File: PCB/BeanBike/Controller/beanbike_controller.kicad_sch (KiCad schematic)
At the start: 16 parts, among them SW1 SW_Push, U4 STM32G473RETx, X1 X49SM8MSD2SC

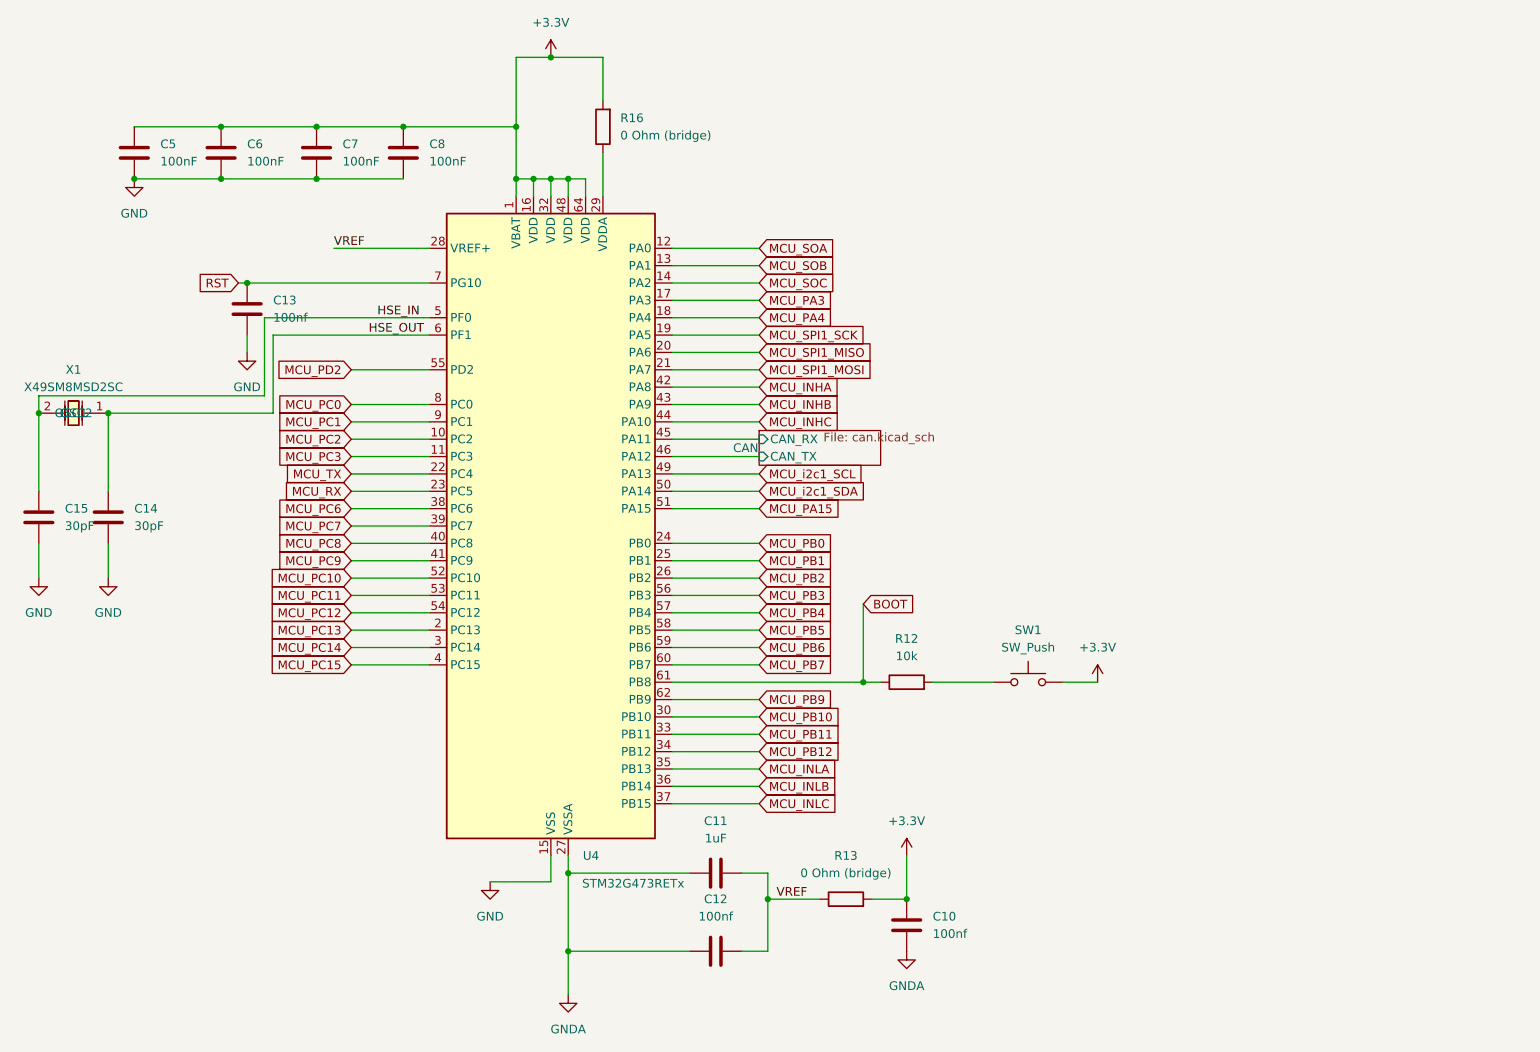
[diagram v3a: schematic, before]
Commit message: PCB v3
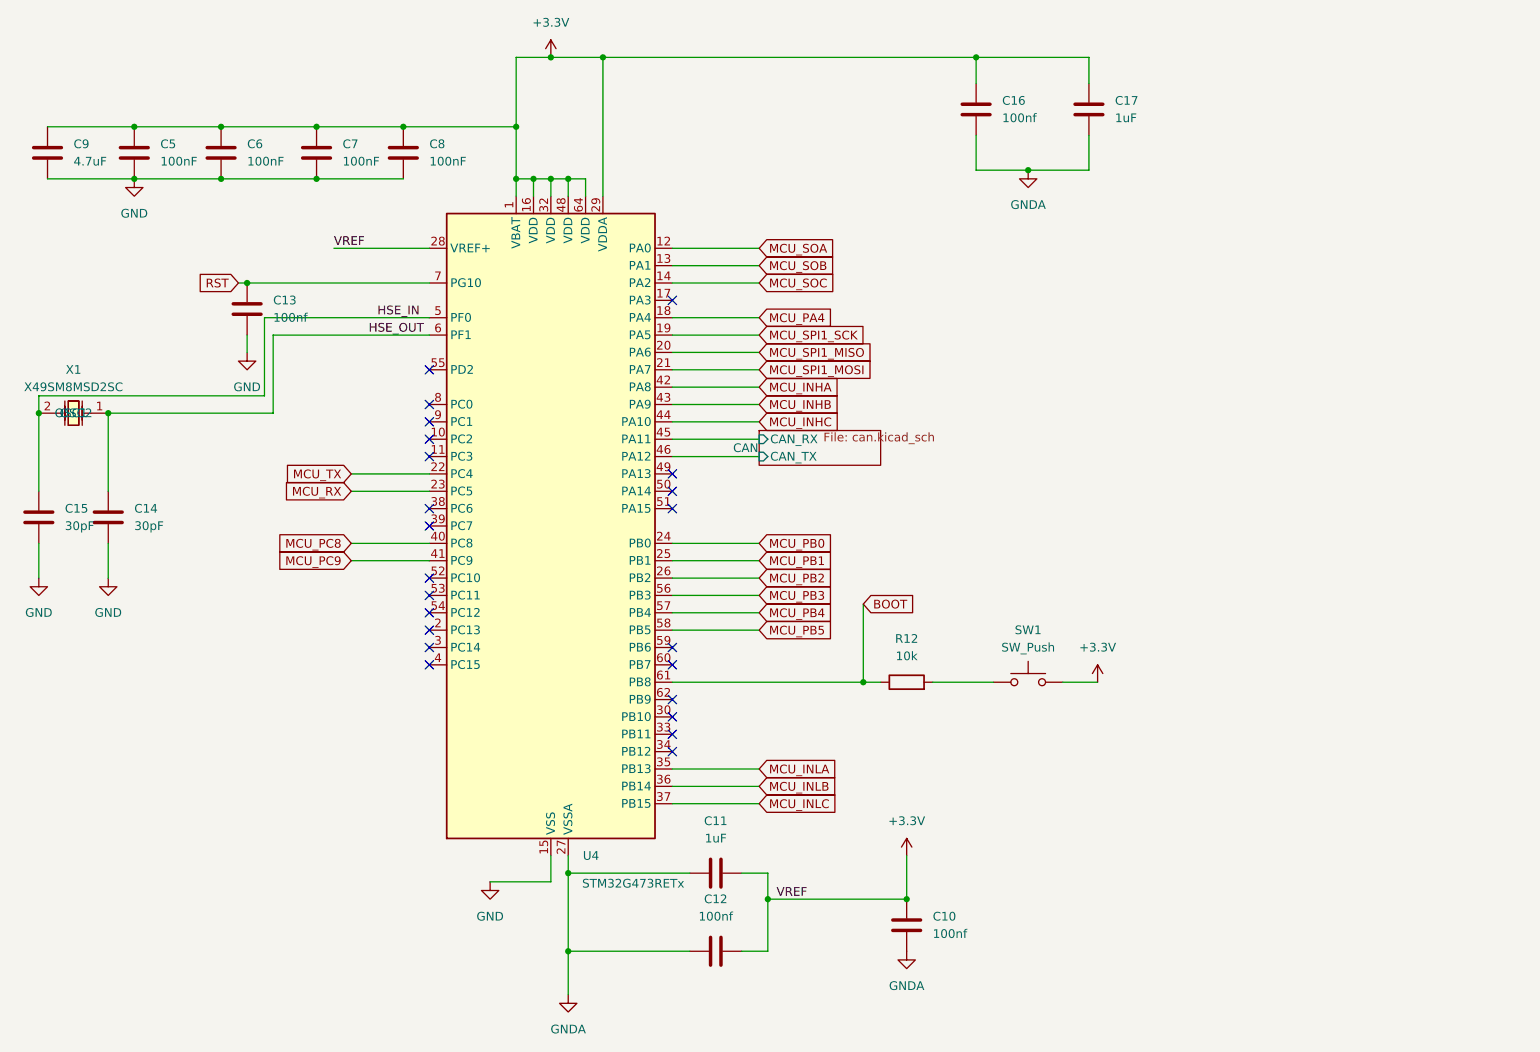
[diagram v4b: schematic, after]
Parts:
- removed R13, R16: 0 Ohm (bridge), Resistor_SMD:R_0805_2012Metric, symbol Device:R
- added C16: 100nf, Capacitor_SMD:C_0402_1005Metric, symbol Device:C
- added C17: 1uF, Capacitor_SMD:C_0402_1005Metric, symbol Device:C
- added C9: 4.7uF, Capacitor_SMD:C_0402_1005Metric, symbol Device:C
- U4: LCSC (none) -> C730120
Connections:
- net VREF is gone; now on net +3.3V: C11.2, C12.2, U4.28 (VREF+)
- net +3.3V: now also U4.29 (VDDA), C16.1, C17.1, C9.1
- net GND: now also C9.2
- net GNDA: now also C16.2, C17.2
- net MCU_PA15: no longer names the net of U4.51 (PA15)
- net MCU_PA3: no longer names the net of U4.17 (PA3)
- net MCU_PB10: no longer names the net of U4.30 (PB10)
- net MCU_PB11: no longer names the net of U4.33 (PB11)
- net MCU_PB12: no longer names the net of U4.34 (PB12)
- net MCU_PB6: no longer names the net of U4.59 (PB6)
- net MCU_PB7: no longer names the net of U4.60 (PB7)
- net MCU_PB9: no longer names the net of U4.62 (PB9)
- net MCU_PC0: no longer names the net of U4.8 (PC0)
- net MCU_PC1: no longer names the net of U4.9 (PC1)
- net MCU_PC10: no longer names the net of U4.52 (PC10)
- net MCU_PC11: no longer names the net of U4.53 (PC11)
- net MCU_PC12: no longer names the net of U4.54 (PC12)
- net MCU_PC13: no longer names the net of U4.2 (PC13)
- net MCU_PC14: no longer names the net of U4.3 (PC14)
- net MCU_PC15: no longer names the net of U4.4 (PC15)
- net MCU_PC2: no longer names the net of U4.10 (PC2)
- net MCU_PC3: no longer names the net of U4.11 (PC3)
- net MCU_PC6: no longer names the net of U4.38 (PC6)
- net MCU_PC7: no longer names the net of U4.39 (PC7)
- net MCU_PD2: no longer names the net of U4.55 (PD2)
- net MCU_i2c1_SCL: no longer names the net of U4.49 (PA13)
- net MCU_i2c1_SDA: no longer names the net of U4.50 (PA14)
- no-connect marks 0 -> 23

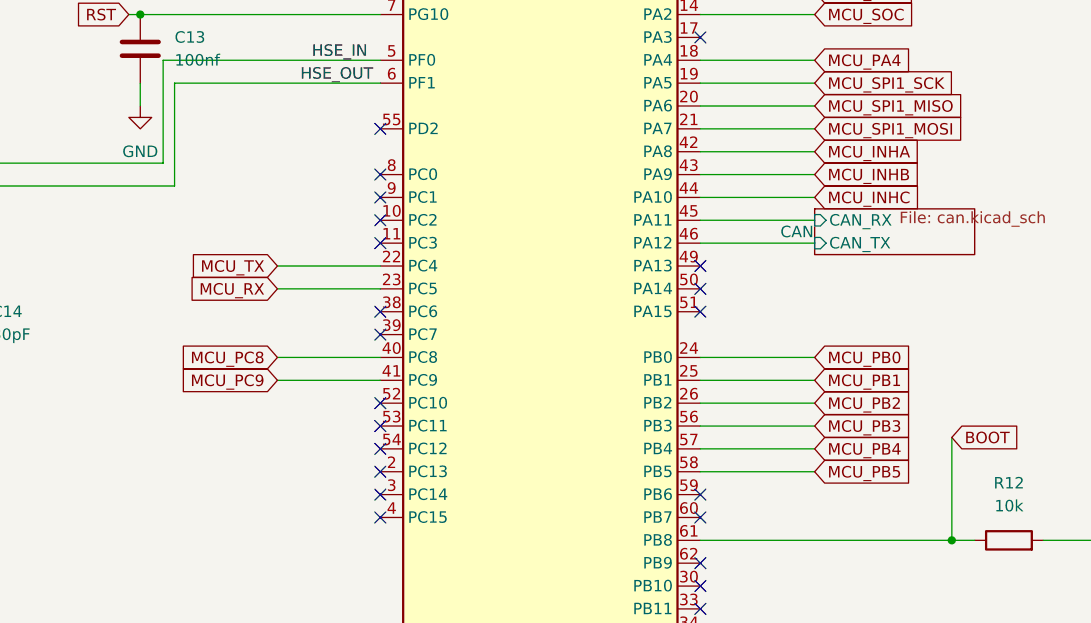
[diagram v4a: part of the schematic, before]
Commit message: PCB v3
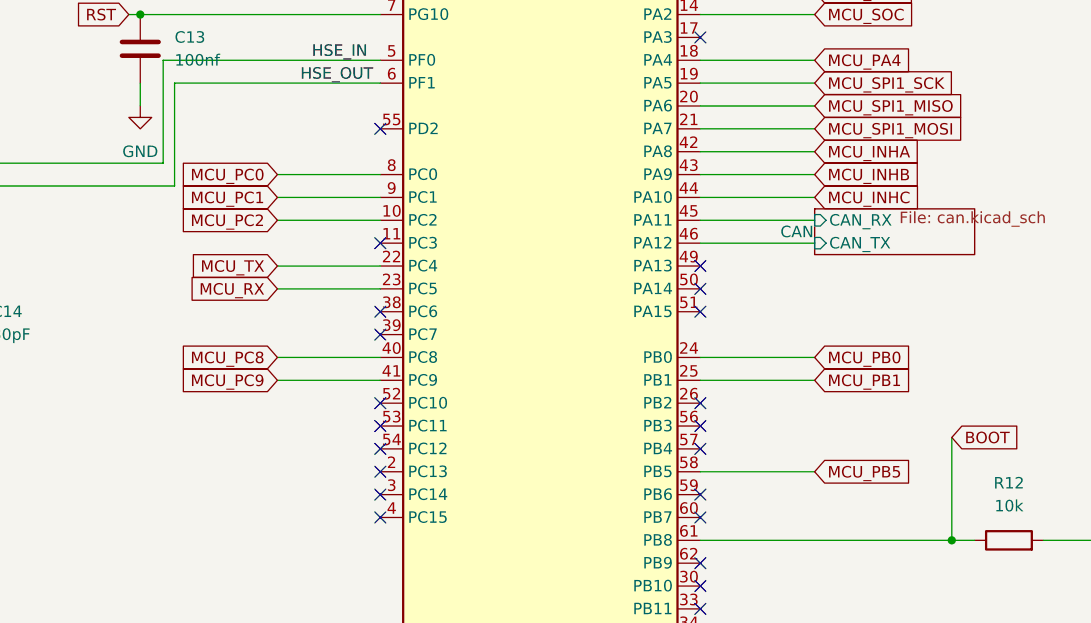
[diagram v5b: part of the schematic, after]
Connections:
- net MCU_PC2: now reaches U4.10 (PC2)
- net MCU_PC0: now reaches U4.8 (PC0)
- net MCU_PC1: now reaches U4.9 (PC1)
- net MCU_PB2: no longer names the net of U4.26 (PB2)
- net MCU_PB3: no longer names the net of U4.56 (PB3)
- net MCU_PB4: no longer names the net of U4.57 (PB4)
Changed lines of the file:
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@@
 	)
 	(no_connect
-		(at 119.38 82.55)
+		(at 154.94 107.95)
+	)
+	(no_connect
+		(at 154.94 110.49)
 	)
 	(no_connect
@@
 	)
 	(no_connect
-		(at 119.38 87.63)
-	)
-	(no_connect
 		(at 154.94 130.81)
 	)
@@
 	)
 	(no_connect
-		(at 119.38 85.09)
+		(at 154.94 113.03)
 	)
 	(no_connect
@@
 	(wire
 		(pts
+			(xy 107.95 82.55) (xy 119.38 82.55)
+		)
+		(stroke
+			(width 0)
+			(type default)
+		)
+	)
+	(wire
+		(pts
 			(xy 168.91 162.56) (xy 168.91 154.94)
 		)
@@
 	(wire
 		(pts
-			(xy 154.94 110.49) (xy 167.64 110.49)
-		)
-		(stroke
-			(width 0)
-			(type default)
-		)
-	)
-	(wire
-		(pts
 			(xy 154.94 140.97) (xy 167.64 140.97)
 		)
@@
 	(wire
 		(pts
+			(xy 107.95 85.09) (xy 119.38 85.09)
+		)
+		(stroke
+			(width 0)
+			(type default)
+		)
+	)
+	(wire
+		(pts
 			(xy 139.7 151.13) (xy 157.48 151.13)
 		)
@@
 	(wire
 		(pts
+			(xy 107.95 87.63) (xy 119.38 87.63)
+		)
+		(stroke
+			(width 0)
+			(type default)
+		)
+	)
+	(wire
+		(pts
 			(xy 134.62 49.53) (xy 132.08 49.53)
 		)
@@
 	(wire
 		(pts
-			(xy 154.94 107.95) (xy 167.64 107.95)
-		)
-		(stroke
-			(width 0)
-			(type default)
-		)
-	)
-	(wire
-		(pts
 			(xy 88.9 49.53) (xy 102.87 49.53)
 		)
@@
 		(pts
 			(xy 132.08 41.91) (xy 132.08 49.53)
-		)
-		(stroke
-			(width 0)
-			(type default)
-		)
-	)
-	(wire
-		(pts
-			(xy 154.94 113.03) (xy 167.64 113.03)
 		)
 		(stroke
@@
 		)
 	)
-	(global_label "MCU_PB3"
-		(shape input)
-		(at 167.64 110.49 0)
-		(fields_autoplaced yes)
-		(effects
-			(font
-				(size 1.27 1.27)
-			)
-			(justify left)
-		)
-		(property "Intersheetrefs" "${INTERSHEET_REFS}"
-			(at 179.3942 110.49 0)
-			(effects
-				(font
-					(size 1.27 1.27)
-				)
-				(justify left)
-				(hide yes)
-			)
-		)
-	)
 	(global_label "MCU_PC8"
 		(shape input)
@@
 		)
 	)
-	(global_label "MCU_PB4"
-		(shape input)
-		(at 167.64 113.03 0)
-		(fields_autoplaced yes)
-		(effects
-			(font
-				(size 1.27 1.27)
-			)
-			(justify left)
-		)
-		(property "Intersheetrefs" "${INTERSHEET_REFS}"
-			(at 179.3942 113.03 0)
-			(effects
-				(font
-					(size 1.27 1.27)
-				)
-				(justify left)
-				(hide yes)
-			)
-		)
-	)
 	(global_label "MCU_INHC"
 		(shape input)
@@
 		)
 	)
+	(global_label "MCU_PC1"
+		(shape input)
+		(at 107.95 85.09 180)
+		(fields_autoplaced yes)
+		(effects
+			(font
+				(size 1.27 1.27)
+			)
+			(justify right)
+		)
+		(property "Intersheetrefs" "${INTERSHEET_REFS}"
+			(at 96.1958 85.09 0)
+			(effects
+				(font
+					(size 1.27 1.27)
+				)
+				(justify right)
+				(hide yes)
+			)
+		)
+	)
 	(global_label "MCU_PC9"
 		(shape input)
@@
 		)
 	)
-	(global_label "MCU_PB2"
-		(shape input)
-		(at 167.64 107.95 0)
-		(fields_autoplaced yes)
-		(effects
-			(font
-				(size 1.27 1.27)
-			)
-			(justify left)
-		)
-		(property "Intersheetrefs" "${INTERSHEET_REFS}"
-			(at 179.3942 107.95 0)
-			(effects
-				(font
-					(size 1.27 1.27)
-				)
-				(justify left)
-				(hide yes)
-			)
-		)
-	)
 	(global_label "MCU_SOB"
 		(shape input)
@@
 		)
 	)
+	(global_label "MCU_PC0"
+		(shape input)
+		(at 107.95 82.55 180)
+		(fields_autoplaced yes)
+		(effects
+			(font
+				(size 1.27 1.27)
+			)
+			(justify right)
+		)
+		(property "Intersheetrefs" "${INTERSHEET_REFS}"
+			(at 96.1958 82.55 0)
+			(effects
+				(font
+					(size 1.27 1.27)
+				)
+				(justify right)
+				(hide yes)
+			)
+		)
+	)
 	(global_label "MCU_RX"
 		(shape input)
@@
 				(hide yes)
 			)
+		)
+	)
+	(global_label "MCU_PC2"
+		(shape input)
+		(at 107.95 87.63 180)
+		(fields_autoplaced yes)
+		(effects
+			(font
+				(size 1.27 1.27)
+			)
+			(justify right)
+		)
+		(property "Intersheetrefs" "${INTERSHEET_REFS}"
+			(at 96.1958 87.63 0)
+			(effects
+				(font
+					(size 1.27 1.27)
+				)
+				(justify right)
+				(hide yes)
+			)

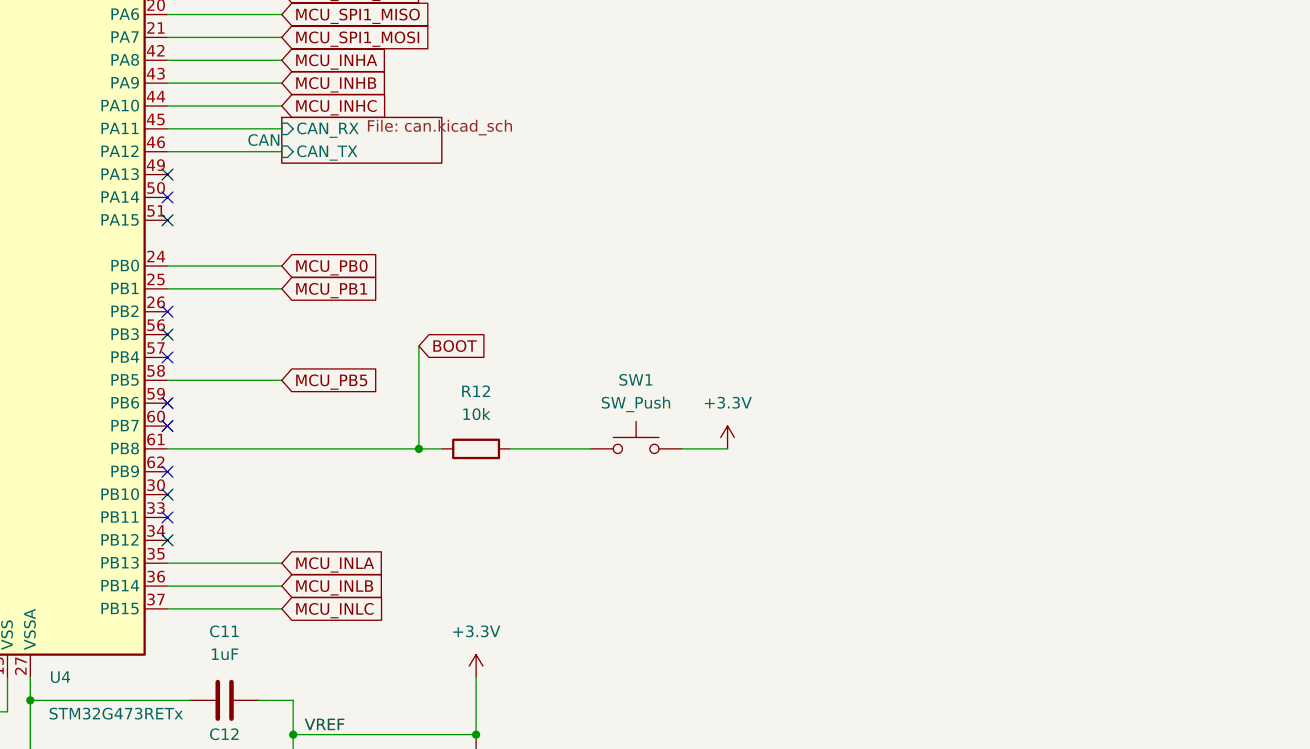
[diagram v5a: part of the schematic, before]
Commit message: big ol update
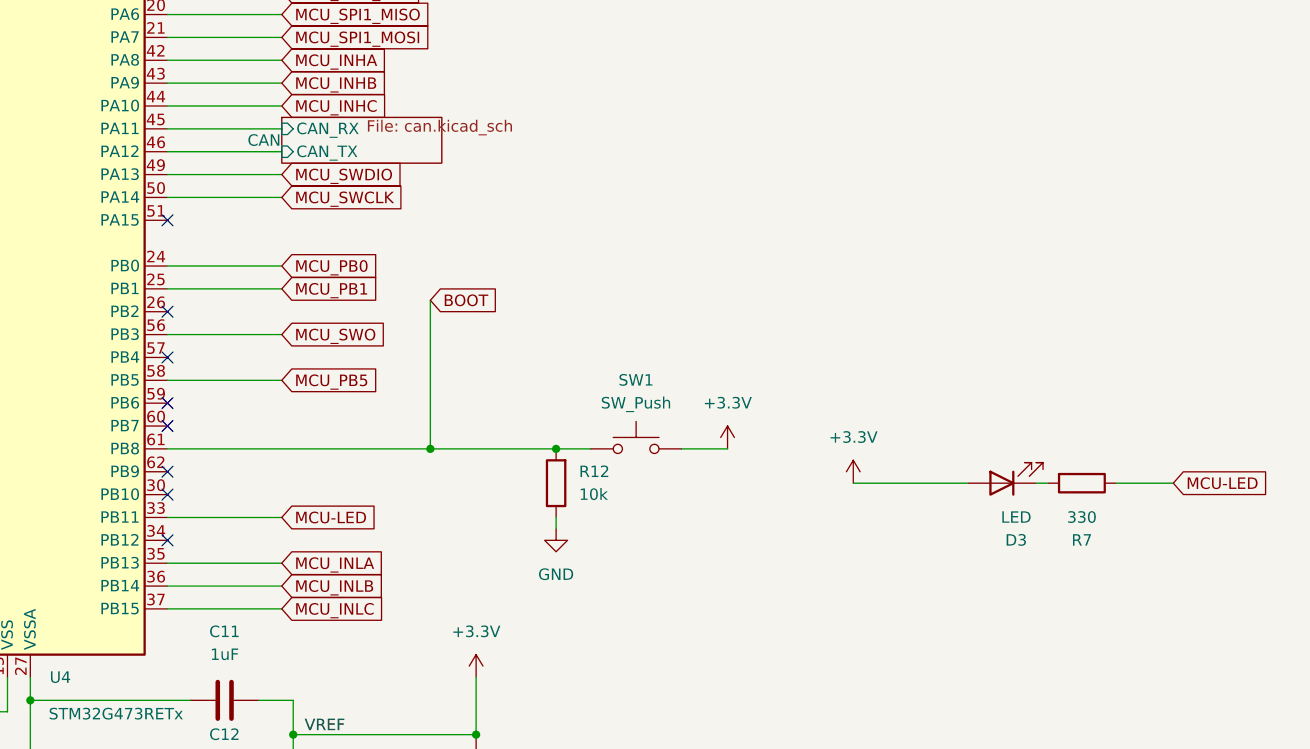
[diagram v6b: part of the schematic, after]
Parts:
- added D3: LED, LED_SMD:LED_0805_2012Metric, symbol Device:LED
- added R7: 330, Resistor_SMD:R_0805_2012Metric, symbol Device:R
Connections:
- net +3.3V: now also D3.2 (A)
- net BOOT: now also R12.2, SW1.1; no longer R12.1
- net GND: now also R12.1
- net MCU-LED: now reaches U4.33 (PB11)
- net MCU-LED: now also R7.1
- net MCU_SWDIO: now reaches U4.49 (PA13)
- net MCU_SWCLK: now reaches U4.50 (PA14)
- net MCU_SWO: now reaches U4.56 (PB3)
- new net: D3.1 (K), R7.2
- no-connect marks 23 -> 19
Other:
- moved on the sheet: R12
